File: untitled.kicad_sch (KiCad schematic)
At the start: 20 parts, among them U10 NCP163ASN180T1G, U11 NCP163ASN330T1G, U7 AP62300WU

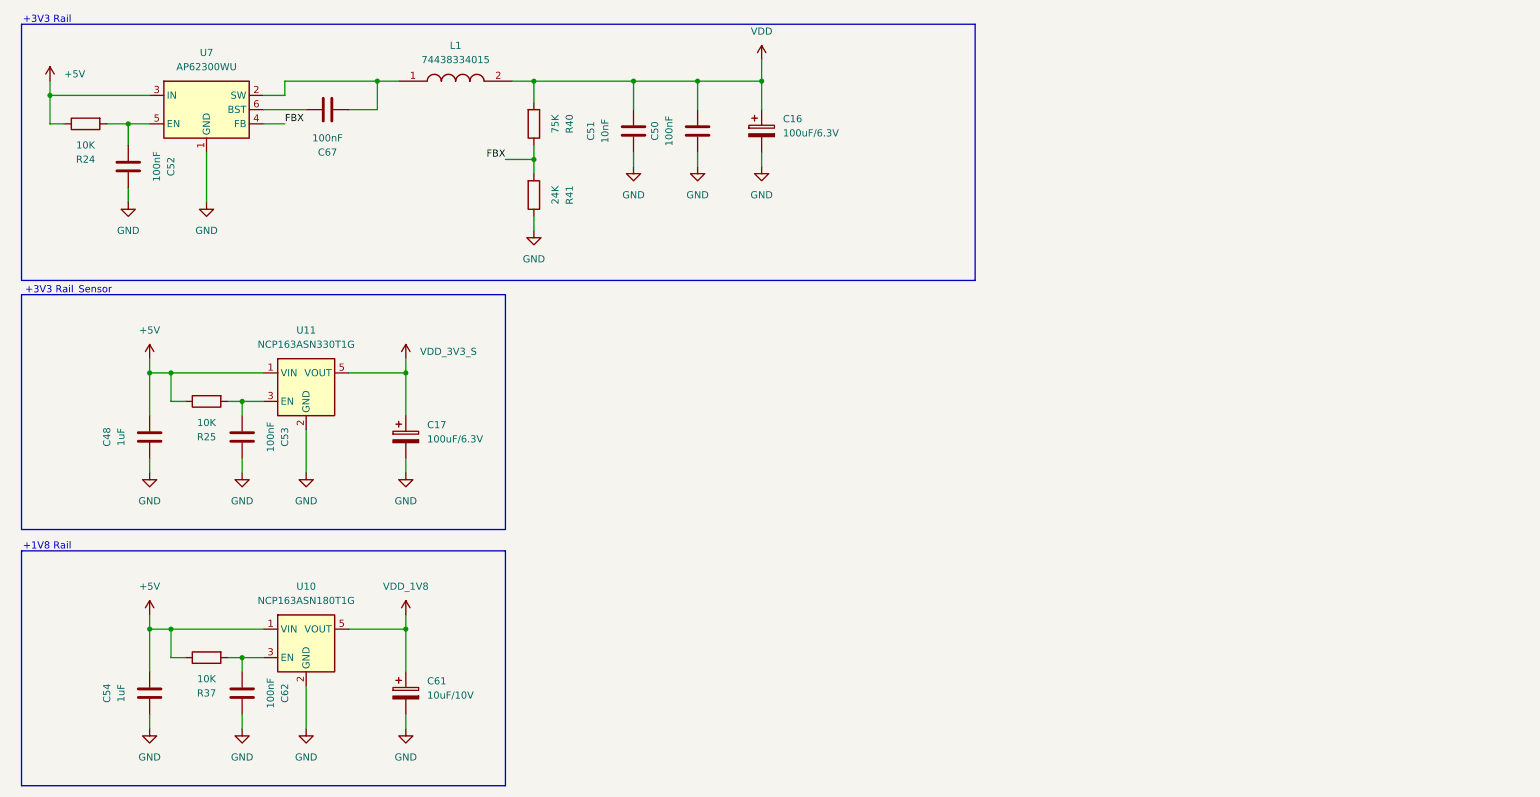
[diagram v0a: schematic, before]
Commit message: Almost Complete Schematic
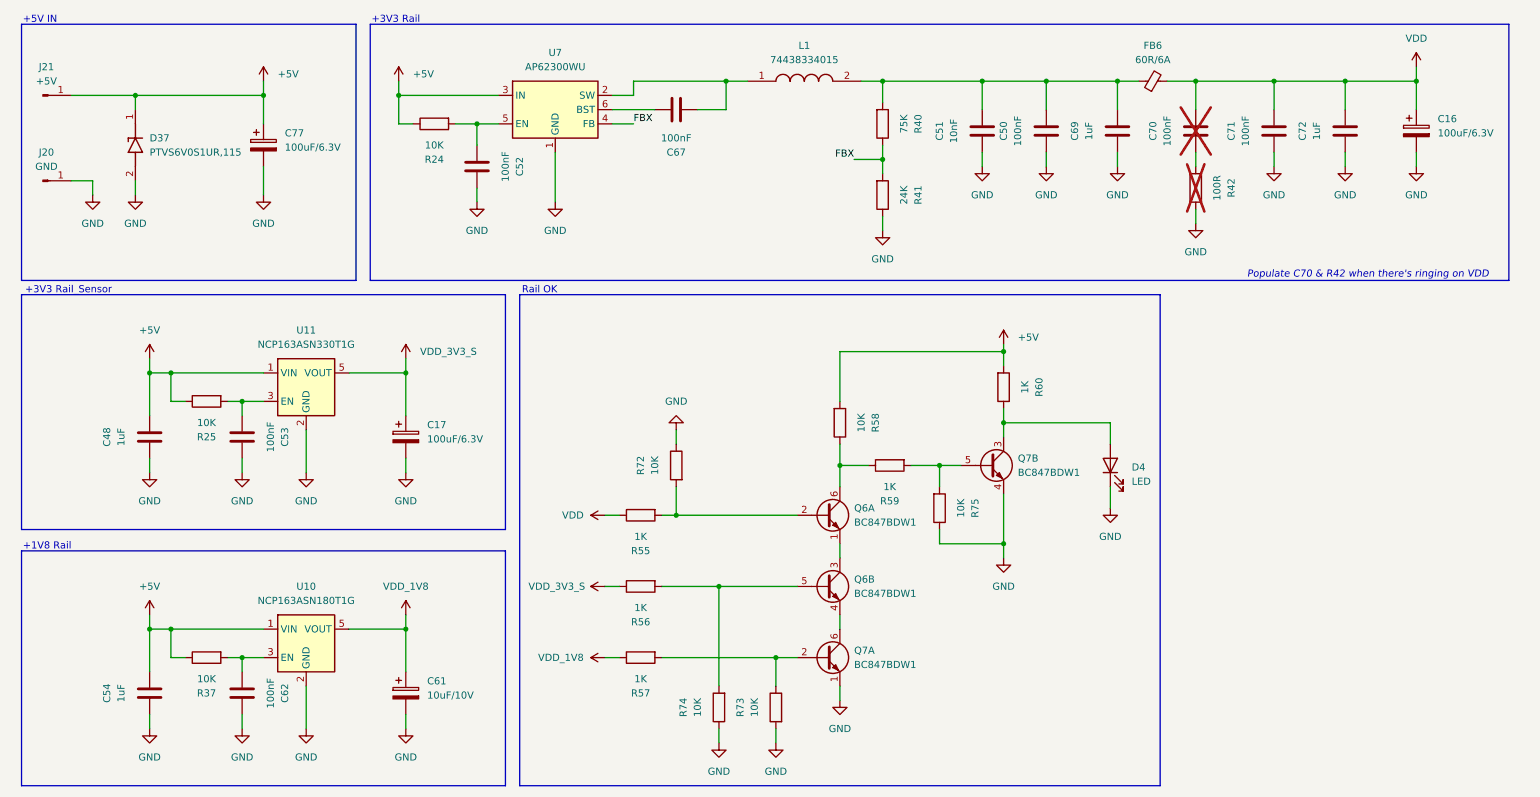
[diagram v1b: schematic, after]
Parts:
- added C69, C72: 1uF, Capacitor_SMD:C_0805_2012Metric, symbol Device:C
- added C70, C71: 100nF, Capacitor_SMD:C_0805_2012Metric, symbol Device:C
- added C77: 100uF/6.3V, Capacitor_Tantalum_SMD:CP_EIA-3528-12_Kemet-T, symbol Device:C_Polarized
- added D37: PTVS6V0S1UR,115, PTVS6V0S1UR:SOD123W, symbol PTVS6V0S1UR_115:PTVS6V0S1UR,115
- added D4: LED, LED_SMD:LED_0805_2012Metric, symbol Device:LED
- added FB6: 60R/6A, Inductor_SMD:L_1806_4516Metric, symbol Device:FerriteBead_Small
- added J20: GND, Connector_Wire:SolderWirePad_1x01_SMD_1.5x3mm, symbol Connector:Conn_01x01_Pin
- added J21: +5V, Connector_Wire:SolderWirePad_1x01_SMD_1.5x3mm, symbol Connector:Conn_01x01_Pin
- added Q6, Q7: BC847BDW1, Package_TO_SOT_SMD:SOT-363_SC-70-6, symbol Transistor_BJT:BC847BDW1
- added R42: 100R, Resistor_SMD:R_0805_2012Metric, symbol Device:R
- added R55, R56, R57, R59, R60: 1K, Resistor_SMD:R_0805_2012Metric, symbol Device:R
- added R58, R72, R73, R74, R75: 10K, Resistor_SMD:R_0805_2012Metric, symbol Device:R
- L1: footprint INDC3030X120N -> WE-74438334015:INDC3030X120N
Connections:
- net +5V: now also C77.1, D37.1 (K), J21.1 (Pin_1), R58.2, R60.2
- net GND: now also C69.1, C71.1, C72.1, C77.2, D37.2 (A), D4.1 (K), J20.1 (Pin_1), Q7.1 (E1), Q7.4 (E2), R42.1, R72.1, R73.2, R74.1, R75.1
- net VDD: now also C70.2, C71.2, C72.2, FB6.2, R55.1; no longer C50.2, C51.2, L1.2, R40.2
- net VDD_1V8: now also R57.1
- net VDD_3V3_S: now also R56.1
- new net: D4.2 (A), Q7.3 (C2), R60.1
- new net: Q7.2 (B1), R57.2, R73.1
- new net: Q6.4 (E2), Q7.6 (C1)
- new net: C50.2, C51.2, C69.2, FB6.1, L1.2, R40.2
- new net: Q6.6 (C1), R58.1, R59.1
- new net: C70.1, R42.2
- new net: Q6.5 (B2), R56.2, R74.2
- new net: Q6.2 (B1), R55.2, R72.2
- new net: Q6.1 (E1), Q6.3 (C2)
- new net: Q7.5 (B2), R59.2, R75.2
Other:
- note added: "+5V IN"
- note added: "Populate C70 & R42 when there's ringing on VDD"
- note added: "Rail OK"
- moved on the sheet: C16, C50, C51, C52, C67, L1, R24, R40, R41, U7
